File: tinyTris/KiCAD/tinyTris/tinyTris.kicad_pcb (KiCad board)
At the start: 2 copper layers, 44.5 x 63.5 mm, 14 parts, among them SW1 Reset, SW2 Rotate, SW3 Left, SW4 Right, SW5 Drop, U1 ATtiny85-20PU, U2 SSD1306_I2C_display

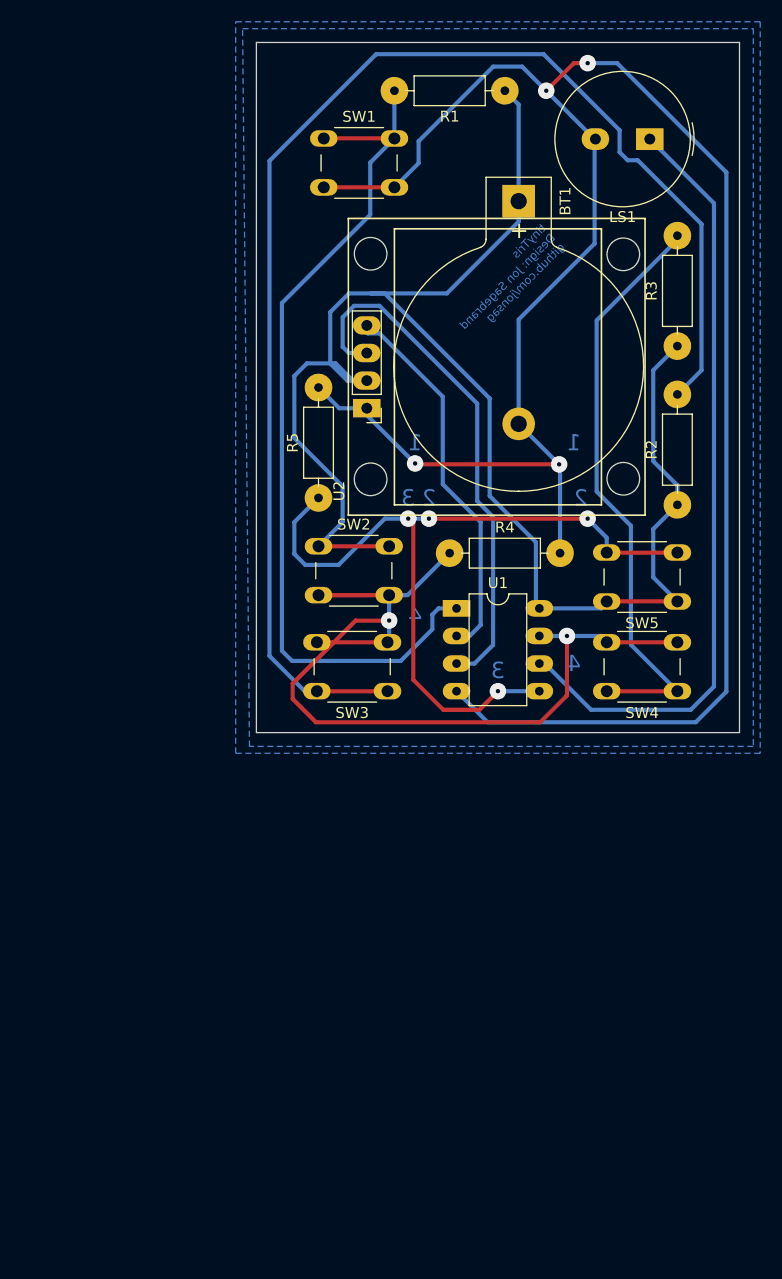
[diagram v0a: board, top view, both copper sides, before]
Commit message: tinyTris Kicad6
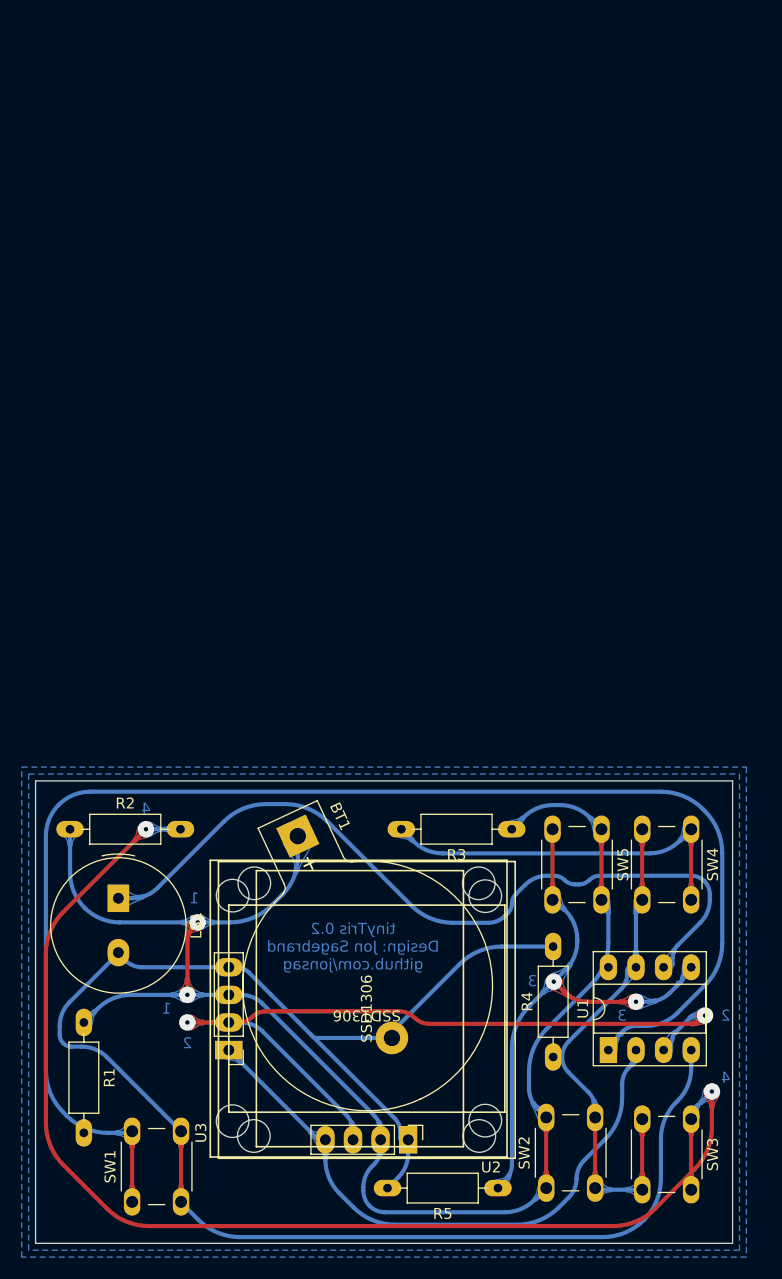
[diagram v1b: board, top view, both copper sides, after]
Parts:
- added U3: SSD1306_I2C_display, My_Parts:SSD1306_I2C_0.96_OLED_display_large, F.Cu at (127.0, 142.2)
- U1: value ATtiny85-20PU -> ATtiny85-20P; footprint My_Misc:DIP-8_W7.62mm_large -> My_Misc:DIP-8_W7.62mm_Socket_w_dip_packet_LongPads
- U2: footprint My_Parts:SSD1306_I2C_0.96_OLED_display_large -> My_Parts:SSD1306_I2C_0.96_OLED_display_no_display_large
- moved SW1 99.4 mm to (118.1, 156.2), turned to 90 degrees
- moved R1 94.1 mm to (113.7, 139.7), turned to -90 degrees
- moved LS1 85.3 mm to (116.8, 128.3), turned to -90 degrees
- moved U2 67.4 mm to (143.5, 150.5), turned to 180 degrees
- moved R5 65.6 mm to (151.8, 154.9), turned to 180 degrees
- moved R2 63.4 mm to (112.4, 121.9), turned to 0 degrees
- moved SW2 62.7 mm to (156.2, 154.9), turned to 90 degrees
- moved BT1 61.9 mm to (133.3, 122.6), turned to -65 degrees
- moved SW3 48.3 mm to (169.5, 148.6), turned to -90 degrees
- moved R4 47.3 mm to (156.8, 142.9), turned to 90 degrees
- moved R3 47.0 mm to (153.0, 121.9), turned to 180 degrees
- moved U1 43.0 mm to (161.9, 142.2), turned to 90 degrees
- moved SW5 22.1 mm to (161.3, 121.9), turned to -90 degrees
- moved SW4 12.8 mm to (169.5, 121.9), turned to -90 degrees
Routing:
- net Net-(R1-Pad2): track 81.6 -> 130.5 mm
- net GND: track 198.1 -> 156.4 mm, vias 4 -> 0
- net Net-(R4-Pad1): track 83.0 -> 49.2 mm, vias 2 -> 0
- net Net-(U2-Pad3): track 48.6 -> 74.2 mm, vias 0 -> 2
- net Net-(R5-Pad1): track 74.1 -> 51.7 mm, vias 4 -> 2
- net Net-(U2-Pad4): track 35.2 -> 55.7 mm
- net Net-(R3-Pad2): track 54.6 -> 34.6 mm
- net Net-(R2-Pad2): track 126.5 -> 117.4 mm, vias 0 -> 2
- net Net-(BT1-Pad1): track 151.2 -> 144.5 mm, vias 0 -> 2
- net Net-(LS1-Pad1): track 71.5 -> 73.6 mm
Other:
- board size 44.5 x 63.5 mm -> 64.1 x 42.5 mm
- net class Default removed
- board text added: "tinyTris 0.2 Design: Jon Sagebrand github.com/jonsag"
- board text removed: "tinyTris Design: Jon Sagebrand github.com/jonsag"
